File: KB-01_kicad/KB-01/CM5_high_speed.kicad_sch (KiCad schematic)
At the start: 2 parts, among them J1 Conn_01x22_MountingPin

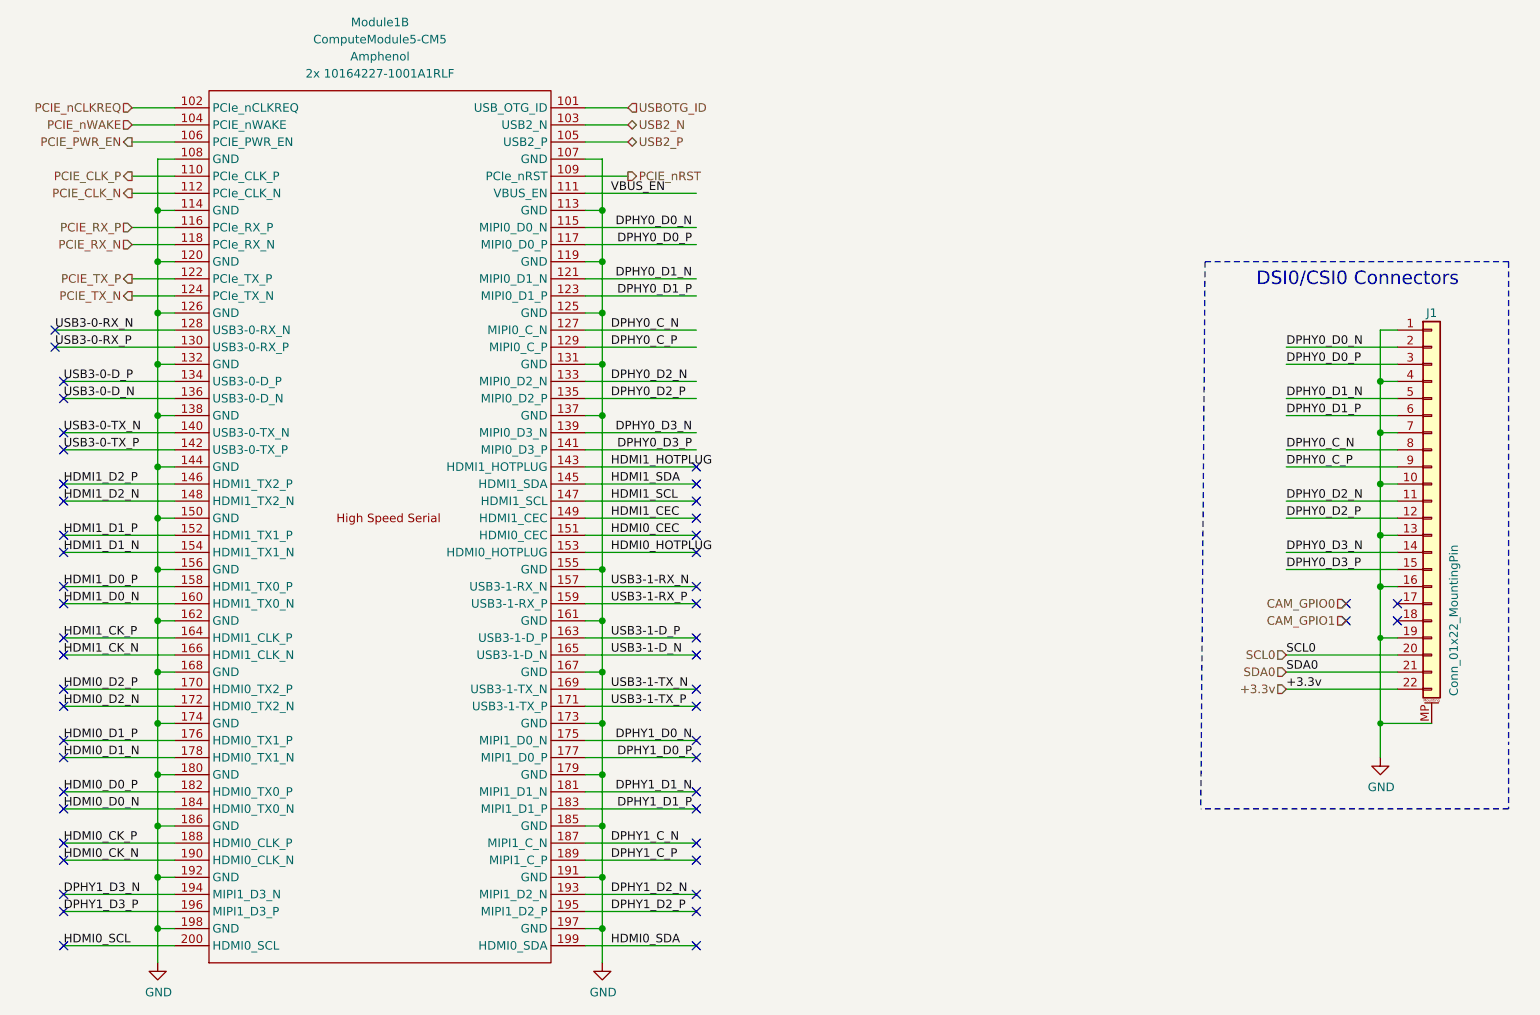
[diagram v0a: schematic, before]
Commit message: all
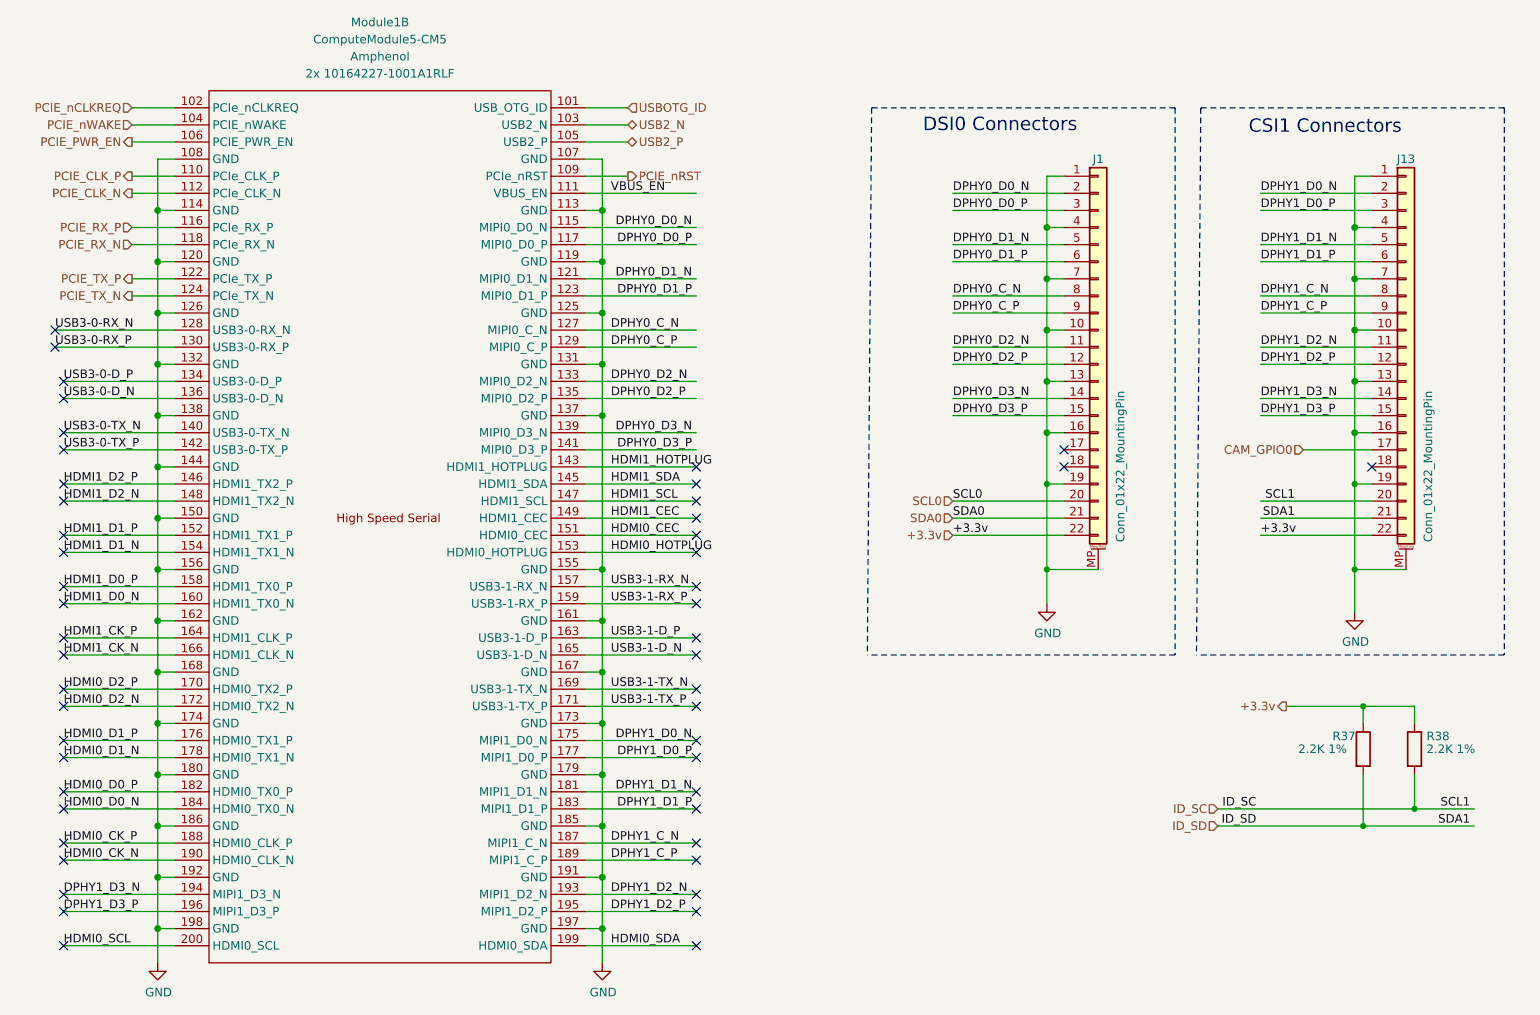
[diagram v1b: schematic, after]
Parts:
- added J13: Conn_01x22_MountingPin, CM5IO:Hirose_FH12-22S-0.5SH_1x22-1MP_P0.50mm_Horizontal, symbol Connector_Generic_MountingPin:Conn_01x22_MountingPin
- added R37, R38: 2.2K 1%, Resistor_SMD:R_0603_1608Metric_Pad0.98x0.95mm_HandSolder, symbol Device:R
- J1: footprint (none) -> CM5IO:Hirose_FH12-22S-0.5SH_1x22-1MP_P0.50mm_Horizontal
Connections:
- net +3.3v: now also J13.22 (Pin_22), R37.1, R38.1
- net CAM_GPIO0: now also J13.17 (Pin_17)
- net DPHY1_C_N: now also J13.8 (Pin_8)
- net DPHY1_C_P: now also J13.9 (Pin_9)
- net DPHY1_D0_N: now also J13.2 (Pin_2)
- net DPHY1_D0_P: now also J13.3 (Pin_3)
- net DPHY1_D1_N: now also J13.5 (Pin_5)
- net DPHY1_D1_P: now also J13.6 (Pin_6)
- net DPHY1_D2_N: now also J13.11 (Pin_11)
- net DPHY1_D2_P: now also J13.12 (Pin_12)
- net DPHY1_D3_N: now also J13.14 (Pin_14)
- net DPHY1_D3_P: now also J13.15 (Pin_15)
- net GND: now also J13.1 (Pin_1), J13.10 (Pin_10), J13.13 (Pin_13), J13.16 (Pin_16), J13.19 (Pin_19), J13.4 (Pin_4), J13.7 (Pin_7), J13.MP (MountPin)
- new net ID_SC: J13.20 (Pin_20), R38.2
- new net ID_SD: J13.21 (Pin_21), R37.2
- no-connect marks 50 -> 49
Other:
- note added: "CSI1 Connectors"
- note added: "DSI0 Connectors"
- note removed: "DSI0/CSI0 Connectors"
- moved on the sheet: J1
